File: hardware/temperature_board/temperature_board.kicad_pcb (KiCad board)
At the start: 2 copper layers, 76 x 20 mm, 13 parts, among them J1 RJ45, U1 TSIC50XF, U2 ST485, m3_loch VAL**

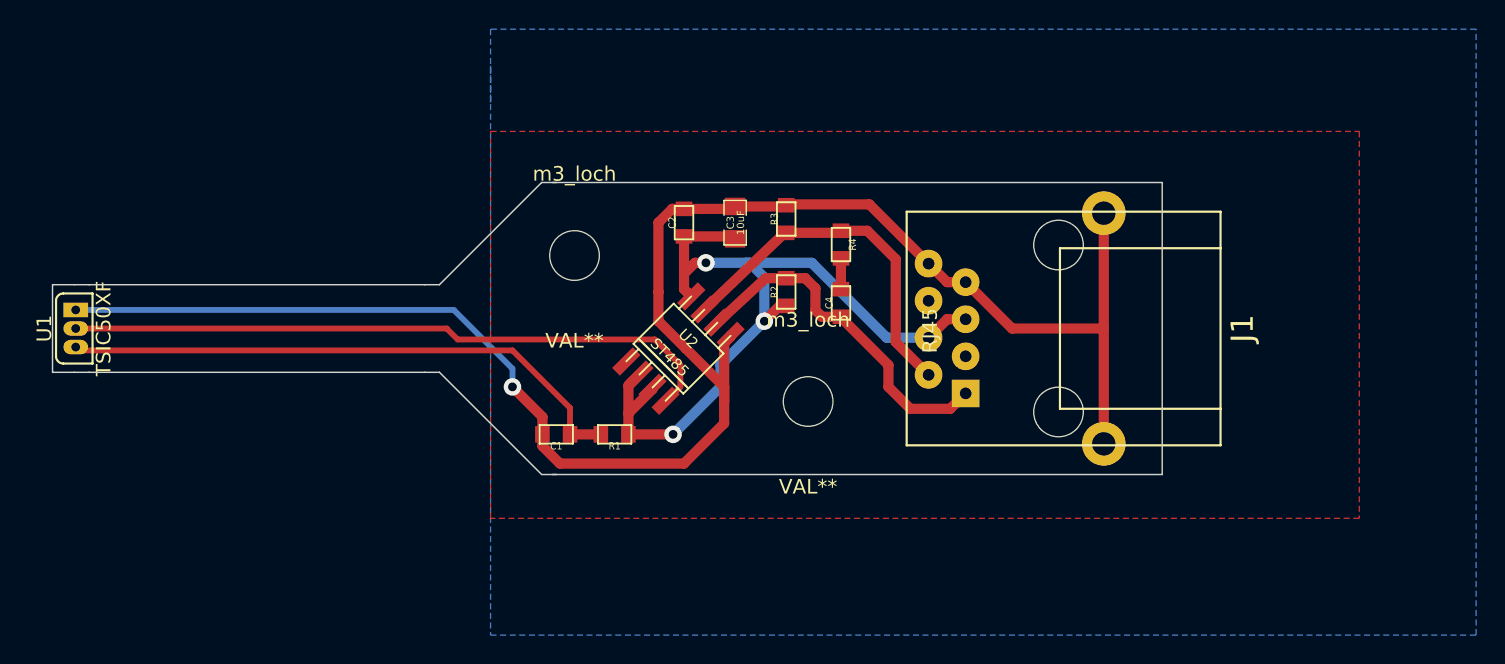
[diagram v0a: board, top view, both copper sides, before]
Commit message: finalized boards for production
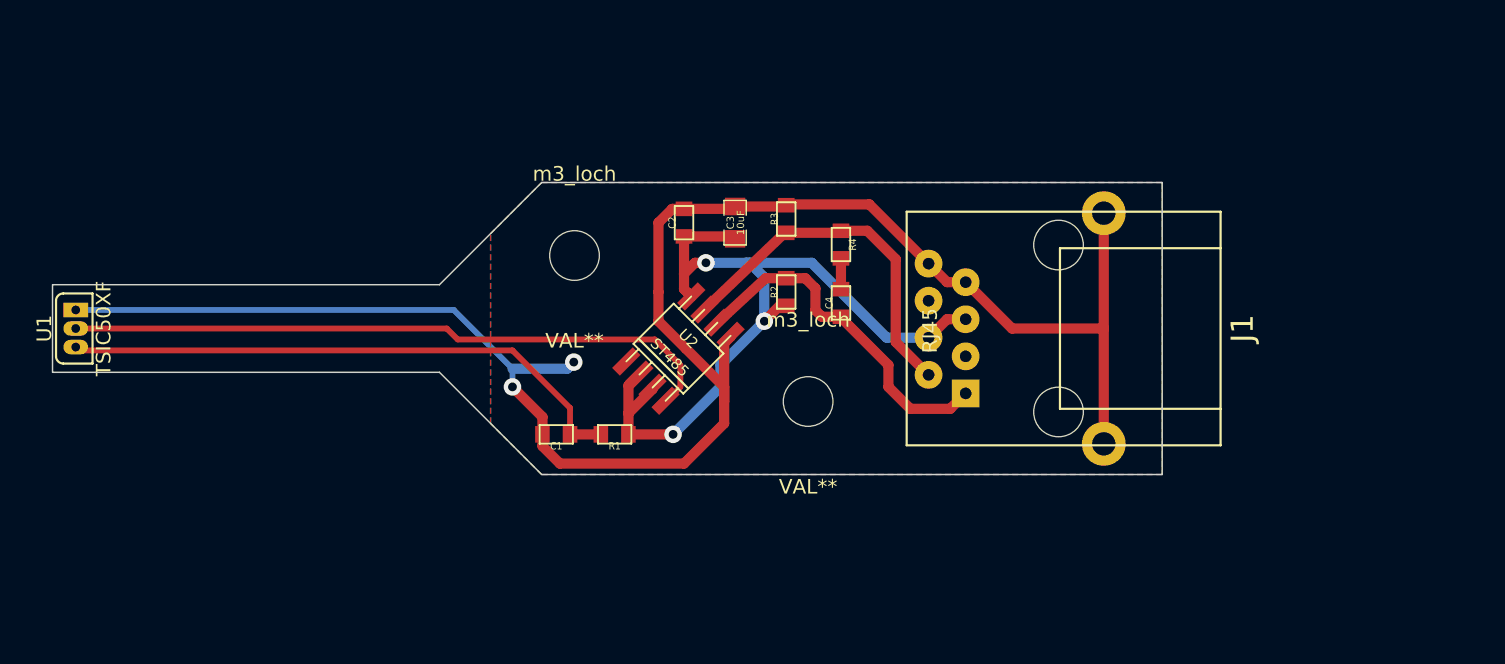
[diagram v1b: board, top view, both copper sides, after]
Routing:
- net GND: track 122.5 -> 126.8 mm, vias 1 -> 2
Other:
- outline, holes or cut-outs redrawn
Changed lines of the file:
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@@
     (links 27)
     (no_connects 0)
-    (area 83.949999 86.949999 176.550001 107.050001)
+    (area 70.214288 75.900001 208.999999 125.2)
     (thickness 1.6)
-    (drawings 23)
-    (tracks 99)
+    (drawings 8)
+    (tracks 102)
     (zones 0)
     (modules 13)
@@
     (pad_to_mask_clearance 0)
     (aux_axis_origin 0 0)
-    (visible_elements FFFFFFFF)
+    (visible_elements 7FFFFFFF)
     (pcbplotparams
       (layerselection 32769)
@@
     )
   )
-  (gr_line (start 160 87) (end 118.25 87) (angle 90) (layer Edge.Cuts) (width 0.1))
   (gr_line (start 160 107) (end 160 87) (angle 90) (layer Edge.Cuts) (width 0.1))
-  (gr_line (start 118.25 107) (end 160 107) (angle 90) (layer Edge.Cuts) (width 0.1))
-  (dimension 4 (width 0.3) (layer Cmts.User)
-    (gr_text "4.000 mm" (at 162 77.400001) (layer Cmts.User)
-      (effects (font (size 1.5 1.5) (thickness 0.3)))
-    )
-    (feature1 (pts (xy 160 88.75) (xy 160 76.050001)))
-    (feature2 (pts (xy 164 88.75) (xy 164 76.050001)))
-    (crossbar (pts (xy 164 78.750001) (xy 160 78.750001)))
-    (arrow1a (pts (xy 160 78.750001) (xy 161.126503 78.163581)))
-    (arrow1b (pts (xy 160 78.750001) (xy 161.126503 79.336421)))
-    (arrow2a (pts (xy 164 78.750001) (xy 162.873497 78.163581)))
-    (arrow2b (pts (xy 164 78.750001) (xy 162.873497 79.336421)))
-  )
-  (dimension 20 (width 0.3) (layer Cmts.User)
-    (gr_text "20.000 mm" (at 202.349999 97.000003 270) (layer Cmts.User)
-      (effects (font (size 1.5 1.5) (thickness 0.3)))
-    )
-    (feature1 (pts (xy 162.5 107) (xy 203.699999 107.000003)))
-    (feature2 (pts (xy 162.5 87) (xy 203.699999 87.000003)))
-    (crossbar (pts (xy 200.999999 87.000003) (xy 200.999999 107.000003)))
-    (arrow1a (pts (xy 200.999999 107.000003) (xy 200.413579 105.8735)))
-    (arrow1b (pts (xy 200.999999 107.000003) (xy 201.586419 105.8735)))
-    (arrow2a (pts (xy 200.999999 87.000003) (xy 200.413579 88.126506)))
-    (arrow2b (pts (xy 200.999999 87.000003) (xy 201.586419 88.126506)))
-  )
-  (dimension 76 (width 0.3) (layer Cmts.User)
-    (gr_text "76.000 mm" (at 122 123.849999) (layer Cmts.User)
-      (effects (font (size 1.5 1.5) (thickness 0.3)))
-    )
-    (feature1 (pts (xy 160 118.25) (xy 160 125.199999)))
-    (feature2 (pts (xy 84 118.25) (xy 84 125.199999)))
-    (crossbar (pts (xy 84 122.499999) (xy 160 122.499999)))
-    (arrow1a (pts (xy 160 122.499999) (xy 158.873497 123.086419)))
-    (arrow1b (pts (xy 160 122.499999) (xy 158.873497 121.913579)))
-    (arrow2a (pts (xy 84 122.499999) (xy 85.126503 123.086419)))
-    (arrow2b (pts (xy 84 122.499999) (xy 85.126503 121.913579)))
-  )
-  (dimension 16 (width 0.3) (layer Cmts.User)
-    (gr_text "16.000 mm" (at 127.75 81.150001) (layer Cmts.User)
-      (effects (font (size 1.5 1.5) (thickness 0.3)))
-    )
-    (feature1 (pts (xy 135.75 102.25) (xy 135.75 79.800001)))
-    (feature2 (pts (xy 119.75 102.25) (xy 119.75 79.800001)))
-    (crossbar (pts (xy 119.75 82.500001) (xy 135.75 82.500001)))
-    (arrow1a (pts (xy 135.75 82.500001) (xy 134.623497 83.086421)))
-    (arrow1b (pts (xy 135.75 82.500001) (xy 134.623497 81.913581)))
-    (arrow2a (pts (xy 119.75 82.500001) (xy 120.876503 83.086421)))
-    (arrow2b (pts (xy 119.75 82.500001) (xy 120.876503 81.913581)))
-  )
-  (gr_line (start 84 100) (end 85.5 100) (angle 90) (layer Edge.Cuts) (width 0.1))
+  (gr_line (start 117.5 107) (end 160 107) (angle 90) (layer Edge.Cuts) (width 0.1))
+  (gr_line (start 110.5 100) (end 117.5 107) (angle 90) (layer Edge.Cuts) (width 0.1))
+  (gr_line (start 84 100) (end 110.5 100) (angle 90) (layer Edge.Cuts) (width 0.1))
   (gr_line (start 84 94) (end 84 100) (angle 90) (layer Edge.Cuts) (width 0.1))
-  (gr_line (start 85.5 94) (end 84 94) (angle 90) (layer Edge.Cuts) (width 0.1))
-  (gr_line (start 109.5 100) (end 110.5 100) (angle 90) (layer Edge.Cuts) (width 0.1))
-  (gr_line (start 110.5 94) (end 109.5 94) (angle 90) (layer Edge.Cuts) (width 0.1))
-  (gr_line (start 117.5 107) (end 118.5 107) (angle 90) (layer Edge.Cuts) (width 0.1))
-  (gr_line (start 110.5 100) (end 117.5 107) (angle 90) (layer Edge.Cuts) (width 0.1))
-  (gr_line (start 117.5 87) (end 118.5 87) (angle 90) (layer Edge.Cuts) (width 0.1))
-  (gr_line (start 110.5 94) (end 117.5 87) (angle 90) (layer Edge.Cuts) (width 0.1))
-  (dimension 6 (width 0.3) (layer Cmts.User)
-    (gr_text "6.000 mm" (at 76.150001 97 270) (layer Cmts.User)
-      (effects (font (size 1.5 1.5) (thickness 0.3)))
-    )
-    (feature1 (pts (xy 85.5 100) (xy 74.800001 100)))
-    (feature2 (pts (xy 85.5 94) (xy 74.800001 94)))
-    (crossbar (pts (xy 77.500001 94) (xy 77.500001 100)))
-    (arrow1a (pts (xy 77.500001 100) (xy 76.913581 98.873497)))
-    (arrow1b (pts (xy 77.500001 100) (xy 78.086421 98.873497)))
-    (arrow2a (pts (xy 77.500001 94) (xy 76.913581 95.126503)))
-    (arrow2b (pts (xy 77.500001 94) (xy 78.086421 95.126503)))
-  )
-  (dimension 25 (width 0.3) (layer Cmts.User)
-    (gr_text "25.000 mm" (at 98 81.650001) (layer Cmts.User)
-      (effects (font (size 1.5 1.5) (thickness 0.3)))
-    )
-    (feature1 (pts (xy 110.5 97) (xy 110.5 80.300001)))
-    (feature2 (pts (xy 85.5 97) (xy 85.5 80.300001)))
-    (crossbar (pts (xy 85.5 83.000001) (xy 110.5 83.000001)))
-    (arrow1a (pts (xy 110.5 83.000001) (xy 109.373497 83.586421)))
-    (arrow1b (pts (xy 110.5 83.000001) (xy 109.373497 82.413581)))
-    (arrow2a (pts (xy 85.5 83.000001) (xy 86.626503 83.586421)))
-    (arrow2b (pts (xy 85.5 83.000001) (xy 86.626503 82.413581)))
-  )
-  (gr_line (start 85.5 94) (end 86.5 94) (angle 90) (layer Edge.Cuts) (width 0.1))
-  (gr_line (start 86.5 100) (end 85.5 100) (angle 90) (layer Edge.Cuts) (width 0.1))
-  (gr_line (start 86.5 94) (end 109.5 94) (angle 90) (layer Edge.Cuts) (width 0.1))
-  (gr_line (start 109.5 100) (end 86.5 100) (angle 90) (layer Edge.Cuts) (width 0.1))
-  (gr_line (start 185 97) (end 87.5 97) (angle 90) (layer Cmts.User) (width 0.2))
+  (gr_line (start 110.5 94) (end 84 94) (angle 90) (layer Edge.Cuts) (width 0.1))
+  (gr_line (start 117.5 87) (end 110.5 94) (angle 90) (layer Edge.Cuts) (width 0.1))
+  (gr_line (start 160 87) (end 117.5 87) (angle 90) (layer Edge.Cuts) (width 0.1))
   (segment (start 138 96.195) (end 138 96.25) (width 0.7) (layer F.Cu) (net 1))
   (segment (start 145.485 102.5) (end 146.54 101.445) (width 0.7) (layer F.Cu) (net 1))
@@
   (segment (start 134.25 90.445) (end 137.86 90.445) (width 0.7) (layer F.Cu) (net 2))
   (segment (start 137.86 90.445) (end 138 90.305) (width 0.7) (layer F.Cu) (net 2))
+  (segment (start 115.5 99.75) (end 119.25 99.75) (width 0.7) (layer B.Cu) (net 3))
+  (via (at 119.7 99.3) (size 1.2) (layers F.Cu B.Cu) (net 3))
+  (segment (start 119.25 99.75) (end 119.7 99.3) (width 0.7) (layer B.Cu) (net 3))
   (segment (start 156 97) (end 149.715 97) (width 0.7) (layer F.Cu) (net 3))
   (segment (start 149.715 97) (end 146.54 93.825) (width 0.7) (layer F.Cu) (net 3))
@@
     (polygon
       (pts
-        (xy 173.5 110) (xy 114 110) (xy 114 83.5) (xy 173.5 83.5)
+        (xy 160 107) (xy 117.5 107) (xy 114 103.5) (xy 114 90.5) (xy 117.5 87)
+        (xy 160 87)
       )
     )
@@
     (polygon
       (pts
-        (xy 114 79) (xy 114 118) (xy 181.5 118) (xy 181.5 76.5) (xy 114 76.5)
-        (xy 114 81.5)
+        (xy 160 107) (xy 117.5 107) (xy 114 103.5) (xy 114 90.5) (xy 117.5 87)
+        (xy 160 87)
       )
     )

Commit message: for put all together
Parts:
- moved U1 418.9 mm to (501.5, 33.0), turned to 180 degrees
- moved m3_loch 387.7 mm to (506.5, 65.2), turned to 270 degrees
- moved C2 381.9 mm to (508.8, 72.8), turned to 0 degrees
- moved C3 378.2 mm to (508.8, 76.2), turned to 0 degrees
- moved C1 377.9 mm to (494.2, 64.0), turned to 90 degrees
- moved R3 374.9 mm to (509.0, 79.8), turned to 0 degrees
- moved U2 374.0 mm to (501.5, 73.8), turned to 225 degrees
- moved R1 373.5 mm to (494.2, 68.0), turned to 90 degrees
- moved R2 370.0 mm to (504.0, 79.8), turned to 0 degrees
- moved R4 369.3 mm to (507.2, 83.5), turned to 180 degrees
- moved C4 365.4 mm to (503.2, 83.5), turned to 0 degrees
- moved m3_loch 361.3 mm to (496.5, 81.2), turned to 270 degrees
- moved J1 357.6 mm to (501.5, 89.5), turned to 180 degrees
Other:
- board size 76 x 20 mm -> 20 x 76 mm
